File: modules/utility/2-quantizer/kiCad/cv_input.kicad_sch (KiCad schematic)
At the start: 7 parts, among them J5 CV_INPUT, U5 TL072, U7 MCP6002

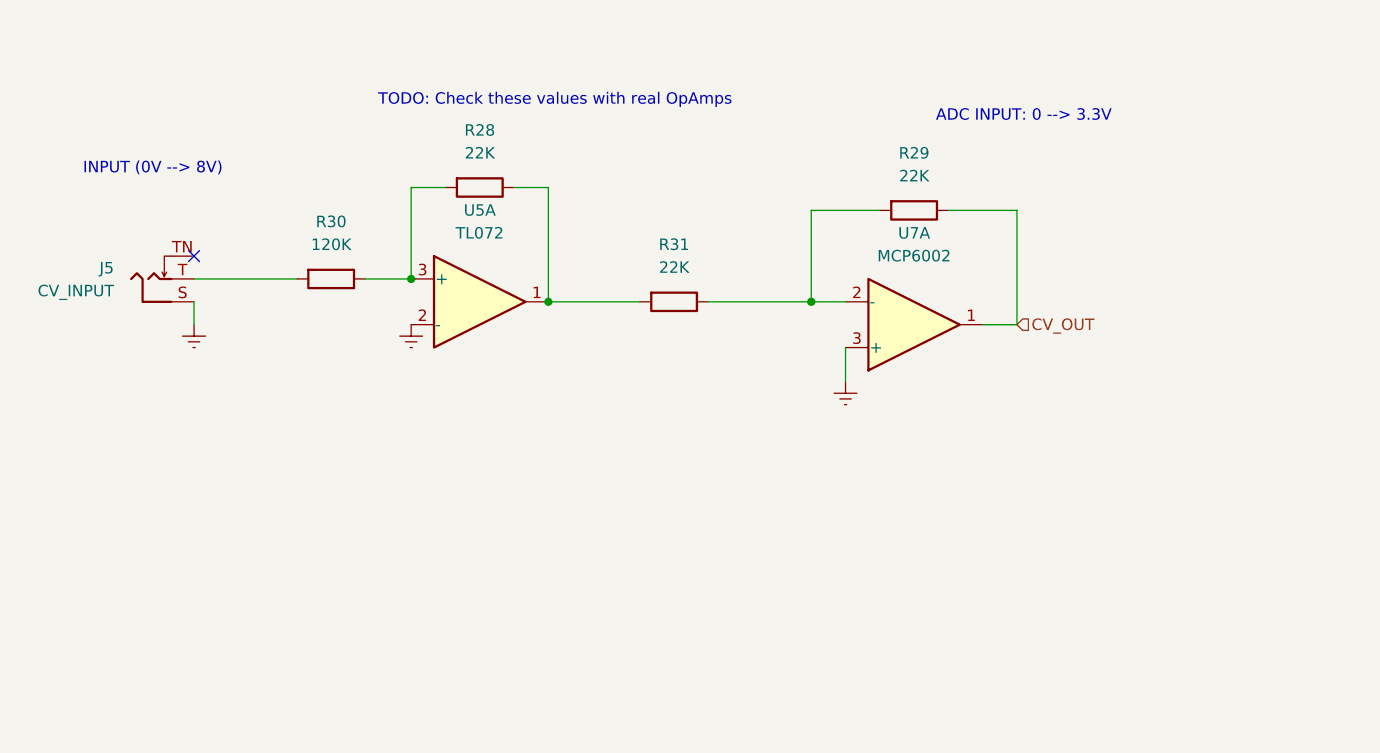
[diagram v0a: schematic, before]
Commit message: quantizers_stls
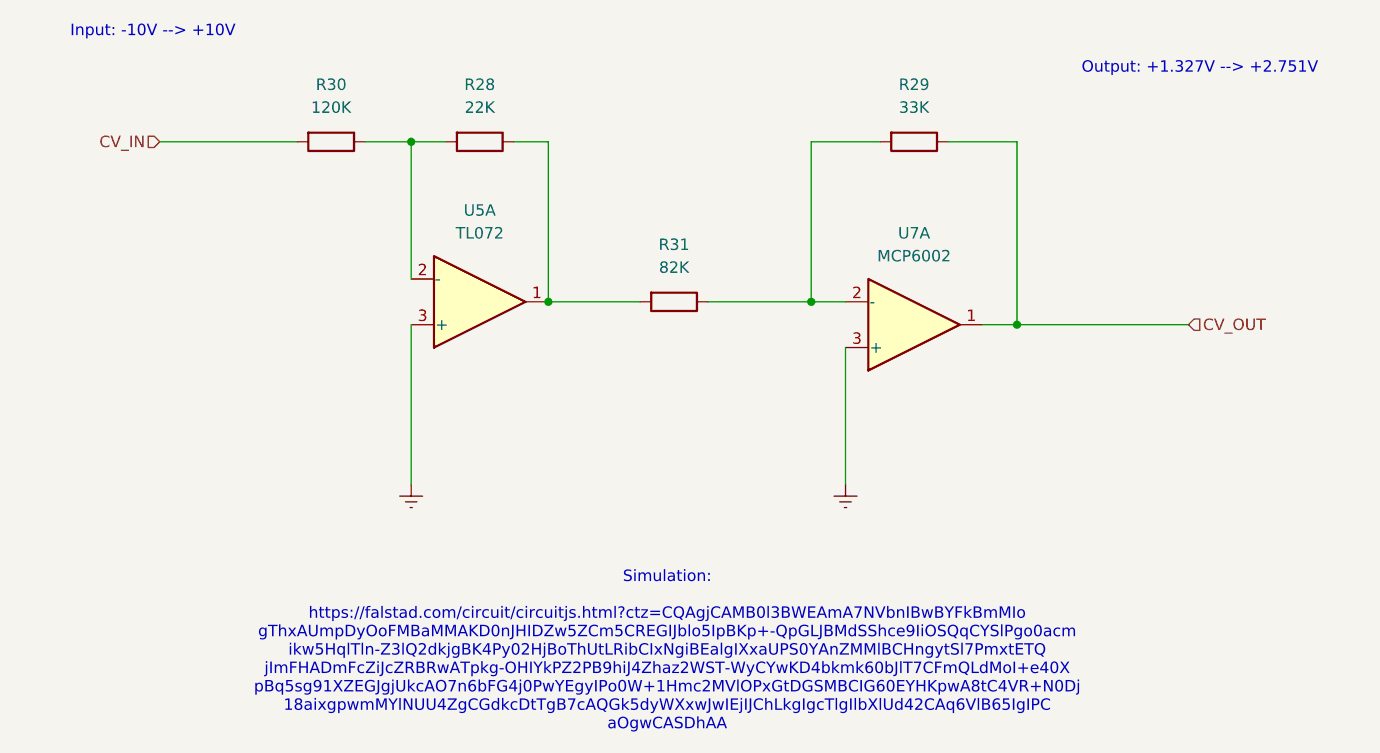
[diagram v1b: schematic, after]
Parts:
- removed J5: CV_INPUT, Synth:Jack_3.5mm_QingPu_WQP-PJ398SM_Vertical_CircularHoles, symbol synth:AudioJack_Mono_3.5mm
- R29: value 22K -> 33K
- R31: value 22K -> 82K
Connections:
- net GNDREF: now also U5.3 (+); no longer U5.2 (-)
- net at R28.2, R30.1: now also U5.2 (-); no longer U5.3 (+)
- net CV_IN: now reaches R30.2
- no-connect marks 1 -> 0
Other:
- note added: "Input: -10V --> +10V"
- note added: "Output: +1.327V --> +2.751V"
- note added: "Simulation: https://falstad.com/circuit/circuitjs.html?ctz=CQAgjCAMB0l3BWEAmA7NVbnIBwBYFkBmMIo gThxAUmpDyOoFMBaMMAKD0nJHIDZw5ZCm5CREGIJblo5IpBKp+-QpGLJBMdSShce9IiOSQqCYSlPgo0acm ikw5HqlTln-Z3lQ2dkjgBK4Py02HjBoThUtLRibCIxNgiBEalgIXxaUPS0YAnZMMlBCHngytSl7PmxtETQ jImFHADmFcZiJcZRBRwATpkg-OHIYkPZ2PB9hiJ4Zhaz2WST-WyCYwKD4bkmk60bJlT7CFmQLdMoI+e40X pBq5sg91XZEGJgjUkcAO7n6bFG4j0PwYEgyIPo0W+1Hmc2MVlOPxGtD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"
- note removed: "ADC INPUT: 0 --> 3.3V"
- note removed: "INPUT (0V --> 8V)"
- note removed: "TODO: Check these values with real OpAmps"
- moved on the sheet: R28, R29, R30
